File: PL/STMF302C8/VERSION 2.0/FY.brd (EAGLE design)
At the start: 76 x 76 mm, 71 parts, among them IC1 EN25F40-100GCP-TR, J1 CON-SD-CARD_MICROSD-2908-05, J4 FEMALE 2x3, U1 AS72652-BLGT, U2 AS72653-BLGT, U3 BMP280, U4 AS72651-BLGT, U5 AMS1117-3.3, U6 4MB Flash, U7 MS561101BA03-50, X1 JST-XH-04-PIN-LONG-PAD, Y2 ABM2B-8.000MHZ-10-1-U-T

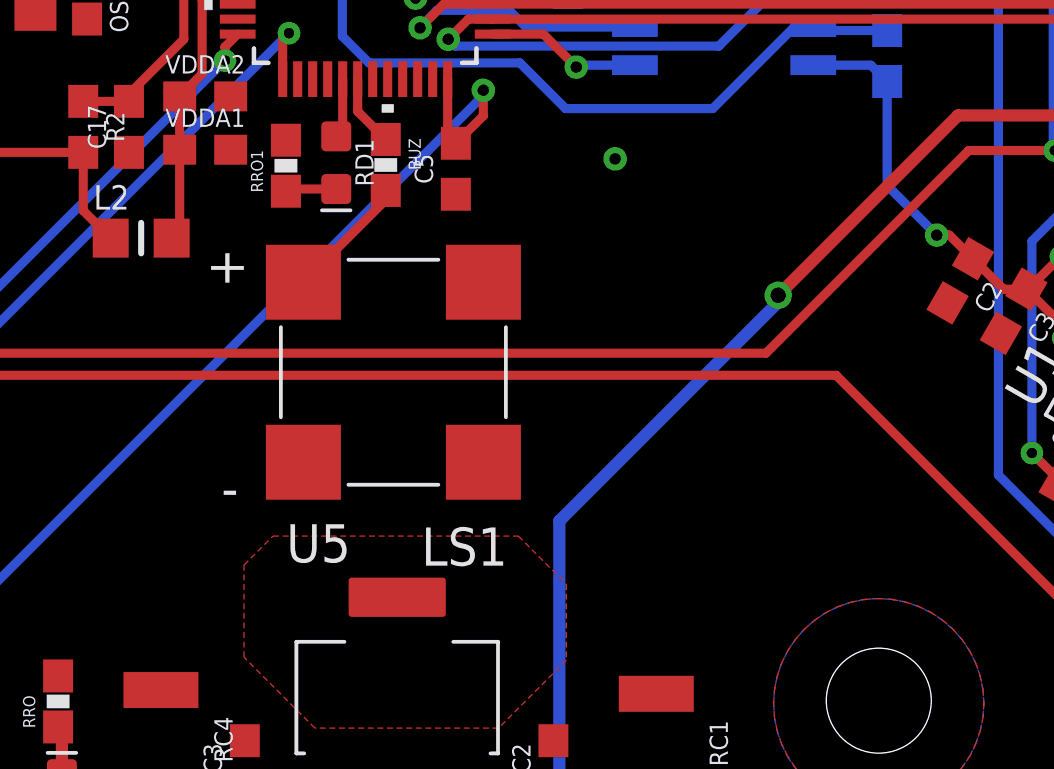
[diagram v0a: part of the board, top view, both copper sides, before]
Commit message: 05.07.2021
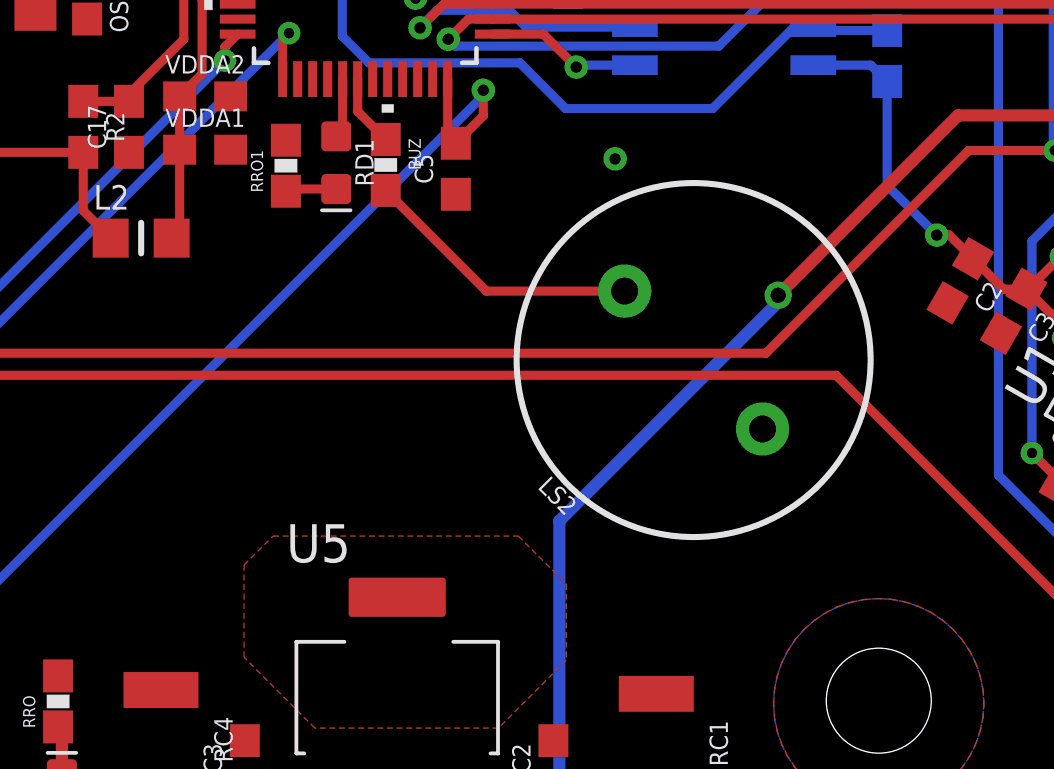
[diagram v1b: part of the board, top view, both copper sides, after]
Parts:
- removed LS1: CMT-7525S-SMT, CMT-7525S-SMT:CUI_CMT-7525S-SMT
- added LS2: BUZZER-PTH, SparkFun-Electromechanical:BUZZER-12MM
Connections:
- net GND: now also LS2.-; no longer LS1.N
- net N$9: now also LS2.+; no longer LS1.P
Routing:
- net N$9: track 4.20 -> 9.35 mm
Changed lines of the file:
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@@
 <attribute name="PURCHASE-URL" value="https://pricing.snapeda.com/search/part/ABM3B-26.000MHZ-10-1-U-T/?ref=eda" x="-10.2616" y="-4.6228" size="1.778" layer="27" rot="R270" display="off"/>
-</element>
-<element name="LS1" library="CMT-7525S-SMT" package="CUI_CMT-7525S-SMT" value="CMT-7525S-SMT" x="44.7802" y="29.1084" smashed="yes" rot="R180">
-<attribute name="AVAILABILITY" value="In Stock" x="44.7802" y="29.1084" size="1.778" layer="27" rot="R180" display="off"/>
-<attribute name="CUI_PURCHASE_URL" value="https://www.cuidevices.com/product/audio/buzzers/audio-transducers/cmt-7525s-smt-tr?utm_source=snapeda.com&amp;utm_medium=referral&amp;utm_campaign=snapedaBOM" x="44.7802" y="29.1084" size="1.778" layer="27" rot="R180" display="off"/>
-<attribute name="DESCRIPTION" value="7.5 mm, 3.6 Vo-p, 90 dB, Surface Mount (SMT), Magnetic Audio Transducer Buzzer" x="44.7802" y="29.1084" size="1.778" layer="27" rot="R180" display="off"/>
-<attribute name="MF" value="CUI Devices" x="44.7802" y="29.1084" size="1.778" layer="27" rot="R180" display="off"/>
-<attribute name="MP" value="CMT-7525S-SMT-TR" x="44.7802" y="29.1084" size="1.778" layer="27" rot="R180" display="off"/>
-<attribute name="NAME" x="48.584709375" y="23.932259375" size="1.271509375" layer="25" rot="R180"/>
-<attribute name="PACKAGE" value=" CUI Inc." x="44.7802" y="29.1084" size="1.778" layer="27" rot="R180" display="off"/>
-<attribute name="PRICE" value="None" x="44.7802" y="29.1084" size="1.778" layer="27" rot="R180" display="off"/>
-<attribute name="VALUE" x="48.59196875" y="35.714940625" size="1.271259375" layer="27" rot="R180"/>
 </element>
 <element name="J2" library="SparkFun-Connectors" library_urn="urn:adsk.eagle:library:513" package="1X05_LOCK_LONGPADS" package3d_urn="urn:adsk.eagle:package:38107/1" value="" x="30.861" y="50.7238" smashed="yes" rot="R90">
@@
 <attribute name="PROD_ID" value="CAP-00868" x="31.3944" y="65.8368" size="1.778" layer="27" rot="R180" display="off"/>
 <attribute name="VALUE" x="23.0632" y="69.8246" size="0.6096" layer="27" font="vector" ratio="20" rot="R180" align="top-center"/>
+</element>
+<element name="LS2" library="SparkFun-Electromechanical" library_urn="urn:adsk.eagle:library:516" package="BUZZER-12MM" package3d_urn="urn:adsk.eagle:package:38558/1" value="BUZZER-PTH" x="54.7878" y="29.5148" smashed="yes" rot="R135">
+<attribute name="NAME" x="50.477278125" y="25.204275" size="0.6096" layer="25" font="vector" ratio="20" rot="R135" align="bottom-center"/>
+<attribute name="PROD_ID" value="COMP-08253" x="54.087340625" y="11.787771875" size="1.778" layer="27" rot="R135" display="off"/>
+<attribute name="SF_SKU" value="COM-07950" x="54.087340625" y="11.787771875" size="1.778" layer="27" rot="R135" display="off"/>
+<attribute name="VALUE" x="50.8364875" y="25.563484375" size="0.6096" layer="27" font="vector" ratio="20" rot="R135" align="top-center"/>
 </element>
 </elements>
@@
 <via x="36.6776" y="49.8348" extent="1-16" drill="0.381"/>
 <via x="43.2816" y="45.1104" extent="1-16" drill="0.381"/>
-<contactref element="LS1" pad="N"/>
 <contactref element="J2" pad="4"/>
 <via x="36.4236" y="51.7398" extent="1-16" drill="0.381"/>
@@
 <wire x1="20.5134" y1="65.2878" x2="20.5134" y2="65.7478" width="0.3048" layer="1"/>
 <wire x1="20.828" y1="64.9732" x2="20.5134" y2="65.2878" width="0.3048" layer="1"/>
+<contactref element="LS2" pad="-"/>
 </signal>
 <signal name="3.3V" class="1">
@@
 <wire x1="72.6948" y1="37.6682" x2="63.6016" y2="37.6682" width="0.4064" layer="1"/>
 </signal>
-<signal name="N$9">
-<contactref element="BUZ" pad="2"/>
-<contactref element="LS1" pad="P"/>
-<wire x1="44.5262" y1="35.1672" x2="44.5262" y2="34.8544" width="0.3048" layer="1"/>
-<wire x1="44.5262" y1="34.8544" x2="41.7802" y2="32.1084" width="0.3048" layer="1"/>
-</signal>
 <signal name="N$3">
 <contactref element="POWER1" pad="2"/>
@@
 <wire x1="49.7781" y1="40.3792" x2="48.0904" y2="40.3792" width="0.3048" layer="1"/>
 </signal>
+<signal name="N$9">
+<contactref element="BUZ" pad="2"/>
+<contactref element="LS2" pad="+"/>
+<wire x1="44.5262" y1="35.1672" x2="47.880503125" y2="31.812896875" width="0.3048" layer="1"/>
+<wire x1="47.880503125" y1="31.812896875" x2="52.4897" y2="31.812896875" width="0.3048" layer="1"/>
+</signal>
 </signals>
